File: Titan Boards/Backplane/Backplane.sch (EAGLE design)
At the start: 29 parts, among them P1 39-30-02_S, P3 39-30-04_S

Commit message: Initial schematic design backplane
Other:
- note added: "3.3V/5V Output Connector"
- note added: "Actuator Connector"
- note added: "Battery Balancer Connector"
- note added: "Coprocessor Connector"
- note added: "ESC Connector"
- note added: "Enable Signals Connector"
- note added: "I2C Control Connector"
- note added: "Kill Switch Connector"
- note added: "Lorem ipsum"
- note added: "Schematic Notes:"
- note added: "Switch Connector"
- note added: "Thurster Signal Connector"

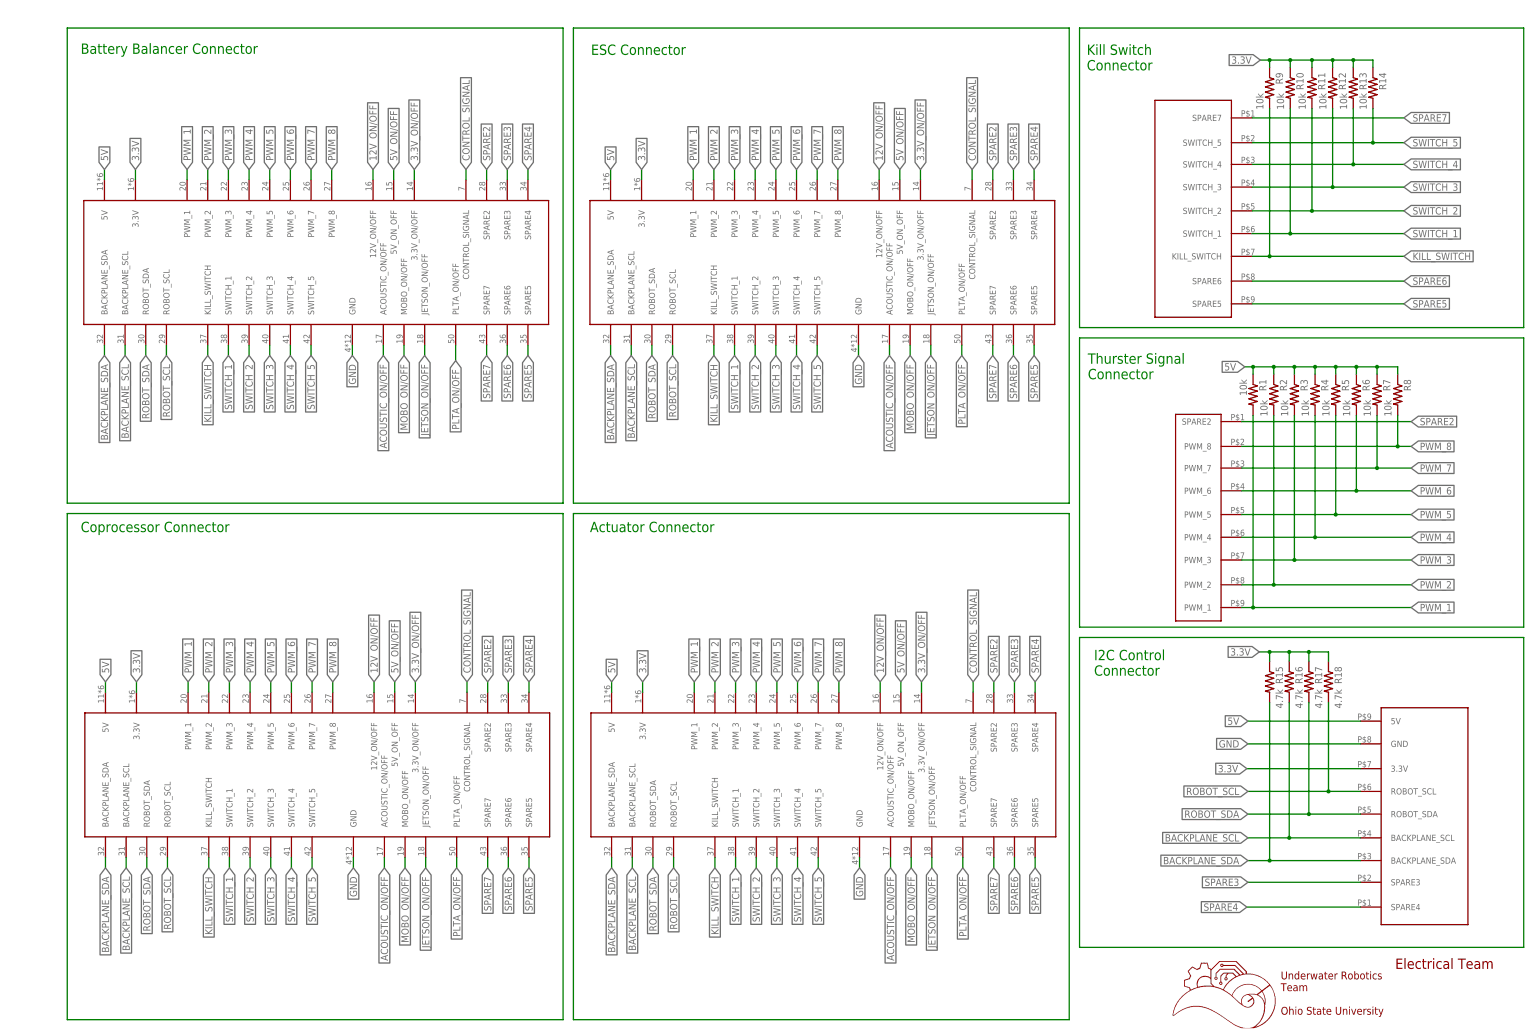
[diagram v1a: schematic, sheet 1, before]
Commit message: First final version of Titan Backplane Schematic
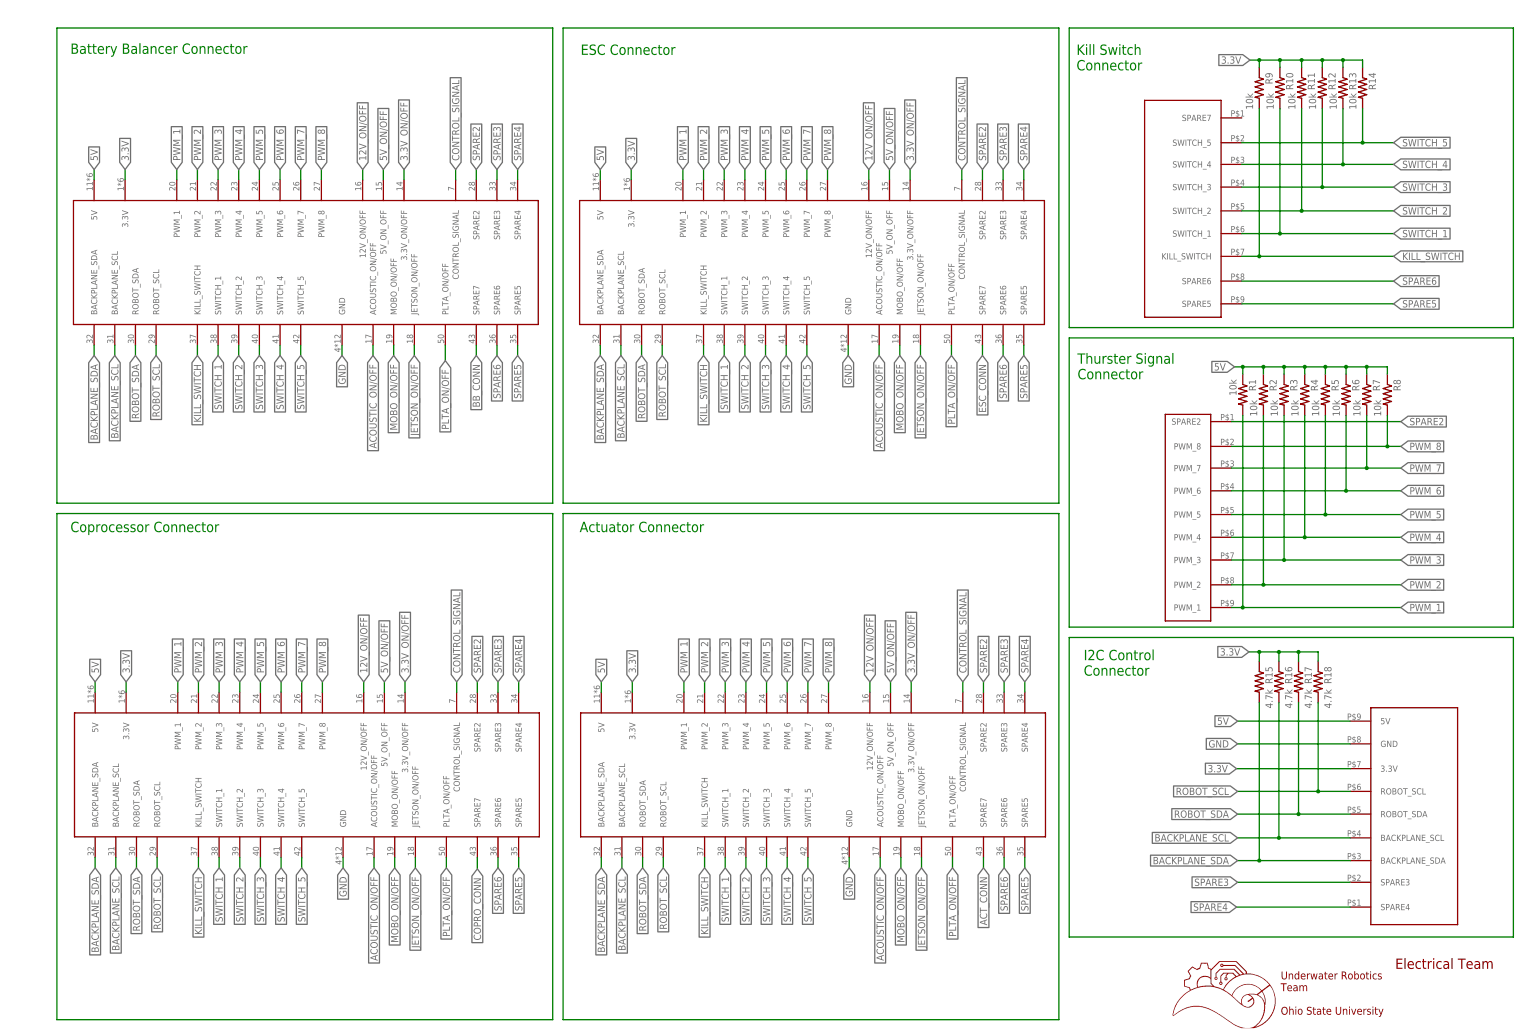
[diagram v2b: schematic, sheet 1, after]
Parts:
- removed P1: 39-30-02_S, con-molex-mini-fit:39-30-02_S
- removed P3: 39-30-04_S, con-molex-mini-fit:39-30-04_S
- removed U$5: 929870-01-09_1, 3M_929852_Connector:929870-01-09_1
- removed U$6: 929870-01-09_2, 3M_929852_Connector:929870-01-09_2
- removed U$8: 929870-01-09_4, 3M_929852_Connector:929870-01-09_4
- added 3.3V_CONNECTOR: 39-30-04_S, con-molex-mini-fit:39-30-04_S
- added 5V_CONNECTOR: 39-30-02_S, con-molex-mini-fit:39-30-02_S
- added ACT_CONN_LED, BB_CONN_LED, COPRO_CONN_LED, ESC_CONN_LED: (no value), led:LEDCHIP-LED0603
- added I2C_CONNECTOR: 929870-01-09_4, 3M_929852_Connector:929870-01-09_4
- added KILLSWITCH_CONNECTOR: 929870-01-09_1, 3M_929852_Connector:929870-01-09_1
- added R19, R20, R21, R22: 36, rcl:R-US_R0603
- added THRUSTER_CONNECTOR: 929870-01-09_2, 3M_929852_Connector:929870-01-09_2
- renumbered U$7 to ENABLE_SIGNALS_CONNECTOR
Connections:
- removed net SPARE7: U$1.SPARE7, U$2.SPARE7, U$3.SPARE7, U$4.SPARE7, U$5.SPARE7
- new net ACT_CONN: ACT_CONN_LED.A, U$4.SPARE7
- new net BB_CONN: BB_CONN_LED.A, U$1.SPARE7
- new net COPRO_CONN: COPRO_CONN_LED.A, U$3.SPARE7
- new net ESC_CONN: ESC_CONN_LED.A, U$2.SPARE7
- new net N$12: BB_CONN_LED.C, R19.1
- new net N$13: ESC_CONN_LED.C, R20.1
- new net N$14: COPRO_CONN_LED.C, R21.1
- new net N$15: ACT_CONN_LED.C, R22.1
- net 3.3V: now also 3.3V_CONNECTOR-1.P, I2C_CONNECTOR.3.3V; no longer P3-1.P, U$8.3.3V
- net 5V: now also 5V_CONNECTOR-1.P, I2C_CONNECTOR.5V; no longer P1-1.P, U$8.5V
- net BACKPLANE_SCL: now also I2C_CONNECTOR.BACKPLANE_SCL; no longer U$8.BACKPLANE_SCL
- net BACKPLANE_SDA: now also I2C_CONNECTOR.BACKPLANE_SDA; no longer U$8.BACKPLANE_SDA
- net GND: now also 3.3V_CONNECTOR-3.P, 5V_CONNECTOR-2.P, I2C_CONNECTOR.GND, R19.2, R20.2, R21.2, R22.2; no longer P1-2.P, P3-3.P, U$8.GND
- net KILL_SWITCH: now also KILLSWITCH_CONNECTOR.KILL_SWITCH; no longer U$5.KILL_SWITCH
- net PWM_1: now also THRUSTER_CONNECTOR.PWM_1; no longer U$6.PWM_1
- net PWM_2: now also THRUSTER_CONNECTOR.PWM_2; no longer U$6.PWM_2
- net PWM_3: now also THRUSTER_CONNECTOR.PWM_3; no longer U$6.PWM_3
- net PWM_4: now also THRUSTER_CONNECTOR.PWM_4; no longer U$6.PWM_4
- net PWM_5: now also THRUSTER_CONNECTOR.PWM_5; no longer U$6.PWM_5
- net PWM_6: now also THRUSTER_CONNECTOR.PWM_6; no longer U$6.PWM_6
- net PWM_7: now also THRUSTER_CONNECTOR.PWM_7; no longer U$6.PWM_7
- net PWM_8: now also THRUSTER_CONNECTOR.PWM_8; no longer U$6.PWM_8
- net ROBOT_SCL: now also 3.3V_CONNECTOR-4.P, I2C_CONNECTOR.ROBOT_SCL; no longer P3-4.P, U$8.ROBOT_SCL
- net ROBOT_SDA: now also 3.3V_CONNECTOR-2.P, I2C_CONNECTOR.ROBOT_SDA; no longer P3-2.P, U$8.ROBOT_SDA
- net SPARE2: now also THRUSTER_CONNECTOR.SPARE2; no longer U$6.SPARE2
- net SPARE3: now also I2C_CONNECTOR.SPARE3; no longer U$8.SPARE3
- net SPARE4: now also I2C_CONNECTOR.SPARE4; no longer U$8.SPARE4
- net SPARE5: now also KILLSWITCH_CONNECTOR.SPARE5; no longer U$5.SPARE5
- net SPARE6: now also KILLSWITCH_CONNECTOR.SPARE6; no longer U$5.SPARE6
- net SWITCH_1: now also KILLSWITCH_CONNECTOR.SWITCH_1; no longer U$5.SWITCH_1
- net SWITCH_2: now also KILLSWITCH_CONNECTOR.SWITCH_2; no longer U$5.SWITCH_2
- net SWITCH_3: now also KILLSWITCH_CONNECTOR.SWITCH_3; no longer U$5.SWITCH_3
- net SWITCH_4: now also KILLSWITCH_CONNECTOR.SWITCH_4; no longer U$5.SWITCH_4
- net SWITCH_5: now also KILLSWITCH_CONNECTOR.SWITCH_5; no longer U$5.SWITCH_5
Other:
- note added: "3.3V/5V Connectors"
- note added: "Administrative Notes: Board Name: Titan Backplane Schematic Creation: 08/2020 Schematic Designer: Dylan Trainor Electrical Lead: Phillip Barker"
- note added: "Board Connected Indicators"
- note added: "Part Notes: Board Connectors: 5530843-6 56 Position Female Connector Non Specified - Dual Edge Gold 0.100 in (2.54mm) Black https://www.digikey.com/product-detail/en/te-connectivity-amp-connectors/5530843-6/A31719-ND/770545 Killswitch Connector: 929870-01-09_1 Thruster Signal Connector: 929870-01-09_2 Enable Signals Connector: 929870-01-09_3 I2C Control Connector: 929870-01-09_4 9 Position Recept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"
- note removed: "3.3V/5V Output Connector"
- note removed: "Lorem ipsum"
- moved on the sheet: R1, R10, R11, R12, R13, R14, R15, R16, R17, R18, R2, R3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

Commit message: Titan Backplane Final Version 1
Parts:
- removed 3.3V_CONNECTOR: 39-30-04_S, con-molex-mini-fit:39-30-04_S
- removed ENABLE_SIGNALS_CONNECTOR: 929870-01-09_3, 3M_929852_Connector:929870-01-09_3
- removed I2C_CONNECTOR: 929870-01-09_4, 3M_929852_Connector:929870-01-09_4
- removed KILLSWITCH_CONNECTOR: 929870-01-09_1, 3M_929852_Connector:929870-01-09_1
- removed R1, R10, R11, R12, R13, R14, R2, R3, R4, R5, R6, R7, R8, R9: 10k, rcl:R-US_R0603
- removed THRUSTER_CONNECTOR: 929870-01-09_2, 3M_929852_Connector:929870-01-09_2
- added AUX_I2C_CONNECTOR1, ROBOT_I2C_CONNECTOR: 39-30-04_S, con-molex-mini-fit:39-30-04_S
- added TESTPIN_CONNECTOR: 929870-01-09_4, 3M_929852_Connector:929870-01-09_4
- SWITCH_CONNECTOR: value 39-30-08_S -> 39-30-02_S; device con-molex-mini-fit:39-30-08_S -> con-molex-mini-fit:39-30-02_S
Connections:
- net 12V_ON/OFF: no longer ENABLE_SIGNALS_CONNECTOR.12V_ON/OFF
- net 3.3V: now also AUX_I2C_CONNECTOR1-1.P, ROBOT_I2C_CONNECTOR-1.P, TESTPIN_CONNECTOR.3.3V; no longer 3.3V_CONNECTOR-1.P, I2C_CONNECTOR.3.3V, R10.1, R11.1, R12.1, R13.1, R14.1, R9.1
- net 3.3V_ON/OFF: no longer ENABLE_SIGNALS_CONNECTOR.3.3V_ON/OFF
- net 5V: now also SWITCH_CONNECTOR-1.P, TESTPIN_CONNECTOR.5V; no longer I2C_CONNECTOR.5V, R1.1, R2.1, R3.1, R4.1, R5.1, R6.1, R7.1, R8.1
- net 5V_ON/OFF: no longer ENABLE_SIGNALS_CONNECTOR.5V_ON/OFF
- net ACOUSTIC_ON/OFF: no longer ENABLE_SIGNALS_CONNECTOR.ACOUSTIC_ON/OFF
- net BACKPLANE_SCL: now also TESTPIN_CONNECTOR.BACKPLANE_SCL; no longer I2C_CONNECTOR.BACKPLANE_SCL
- net BACKPLANE_SDA: now also TESTPIN_CONNECTOR.BACKPLANE_SDA; no longer I2C_CONNECTOR.BACKPLANE_SDA
- net CONTROL_SIGNAL: no longer ENABLE_SIGNALS_CONNECTOR.SPARE1
- net GND: now also AUX_I2C_CONNECTOR1-3.P, ROBOT_I2C_CONNECTOR-3.P, SWITCH_CONNECTOR-2.P, TESTPIN_CONNECTOR.GND; no longer 3.3V_CONNECTOR-3.P, ENABLE_SIGNALS_CONNECTOR.GND, I2C_CONNECTOR.GND, SWITCH_CONNECTOR-5.P
- net JETSON_ON/OFF: no longer ENABLE_SIGNALS_CONNECTOR.JETSON_ON/OFF
- net KILL_SWITCH: no longer KILLSWITCH_CONNECTOR.KILL_SWITCH, R9.2, SWITCH_CONNECTOR-2.P
- net MOBO_ON/OFF: no longer ENABLE_SIGNALS_CONNECTOR.MOBO_ON/OFF
- net PLTA_ON/OFF: no longer ENABLE_SIGNALS_CONNECTOR.SPARE8, SWITCH_CONNECTOR-1.P
- net PWM_1: no longer R1.2, THRUSTER_CONNECTOR.PWM_1
- net PWM_2: no longer R2.2, THRUSTER_CONNECTOR.PWM_2
- net PWM_3: no longer R3.2, THRUSTER_CONNECTOR.PWM_3
- net PWM_4: no longer R4.2, THRUSTER_CONNECTOR.PWM_4
- net PWM_5: no longer R5.2, THRUSTER_CONNECTOR.PWM_5
- net PWM_6: no longer R6.2, THRUSTER_CONNECTOR.PWM_6
- net PWM_7: no longer R7.2, THRUSTER_CONNECTOR.PWM_7
- net PWM_8: no longer R8.2, THRUSTER_CONNECTOR.PWM_8
- net ROBOT_SCL: now also AUX_I2C_CONNECTOR1-4.P, ROBOT_I2C_CONNECTOR-4.P, TESTPIN_CONNECTOR.ROBOT_SCL; no longer 3.3V_CONNECTOR-4.P, I2C_CONNECTOR.ROBOT_SCL
- net ROBOT_SDA: now also AUX_I2C_CONNECTOR1-2.P, ROBOT_I2C_CONNECTOR-2.P, TESTPIN_CONNECTOR.ROBOT_SDA; no longer 3.3V_CONNECTOR-2.P, I2C_CONNECTOR.ROBOT_SDA
- net SPARE2: no longer THRUSTER_CONNECTOR.SPARE2
- net SPARE3: now also TESTPIN_CONNECTOR.SPARE3; no longer I2C_CONNECTOR.SPARE3
- net SPARE4: now also TESTPIN_CONNECTOR.SPARE4; no longer I2C_CONNECTOR.SPARE4
- net SPARE5: no longer KILLSWITCH_CONNECTOR.SPARE5
- net SPARE6: no longer KILLSWITCH_CONNECTOR.SPARE6
- net SWITCH_1: no longer KILLSWITCH_CONNECTOR.SWITCH_1, R10.2, SWITCH_CONNECTOR-3.P
- net SWITCH_2: no longer KILLSWITCH_CONNECTOR.SWITCH_2, R11.2, SWITCH_CONNECTOR-4.P
- net SWITCH_3: no longer KILLSWITCH_CONNECTOR.SWITCH_3, R12.2, SWITCH_CONNECTOR-6.P
- net SWITCH_4: no longer KILLSWITCH_CONNECTOR.SWITCH_4, R13.2, SWITCH_CONNECTOR-7.P
- net SWITCH_5: no longer KILLSWITCH_CONNECTOR.SWITCH_5, R14.2, SWITCH_CONNECTOR-8.P
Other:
- note added: "5V Connector"
- note added: "Auxillary I2C Connector"
- note added: "Part Notes: Board Connectors: 5530843-6 56 Position Female Connector Non Specified - Dual Edge Gold 0.100 in (2.54mm) Black https://www.digikey.com/product-detail/en/te-connectivity-amp-connectors/5530843-6/A31719-ND/770545 Test Pin Connector: 929870-01-09 9 Position Receptacle Connector Through Hole https://www.digikey.com/product-detail/en/3m/929870-01-09-RA/929870-01-09-RA-ND/1239312 Board Con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"
- note added: "Robot I2C Connector"
- note added: "Test Pin Connector"
- note removed: "3.3V/5V Connectors"
- note removed: "Enable Signals Connector"
- note removed: "I2C Control Connector"
- note removed: "Kill Switch Connector"
- note removed: "Part Notes: Board Connectors: 5530843-6 56 Position Female Connector Non Specified - Dual Edge Gold 0.100 in (2.54mm) Black https://www.digikey.com/product-detail/en/te-connectivity-amp-connectors/5530843-6/A31719-ND/770545 Killswitch Connector: 929870-01-09_1 Thruster Signal Connector: 929870-01-09_2 Enable Signals Connector: 929870-01-09_3 I2C Control Connector: 929870-01-09_4 9 Position Recept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"
- note removed: "Thurster Signal Connector"
